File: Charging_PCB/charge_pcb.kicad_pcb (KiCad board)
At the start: 2 copper layers, 96.5 x 50.8 mm, 40 parts, among them J1 PCB_1, J2 Battery, J3 Power Switch, J4 24V Out, J5 Motor_Drive, J6 Motor_Cutter, J7 24V Out, J8 Start, J9 24V out, Q1 BC547C, Q2 IRF9540N, Q3 BC547C, Q4 IRF9540N, U1 INA169

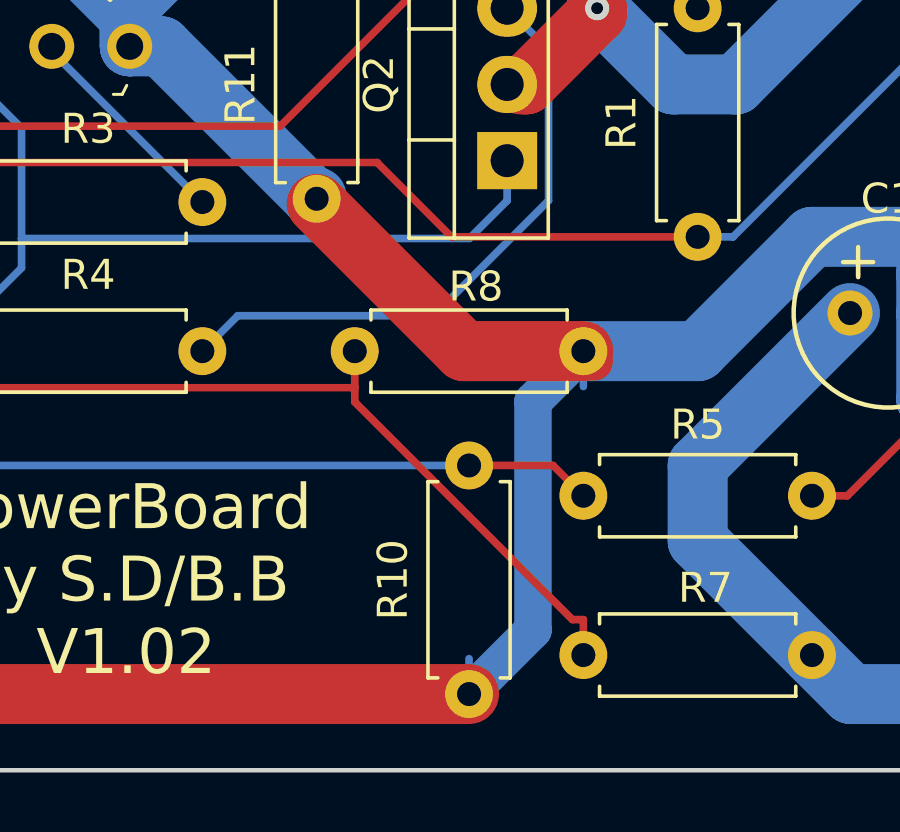
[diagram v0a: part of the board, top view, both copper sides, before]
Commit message: Add Schematic PDF and new Picture
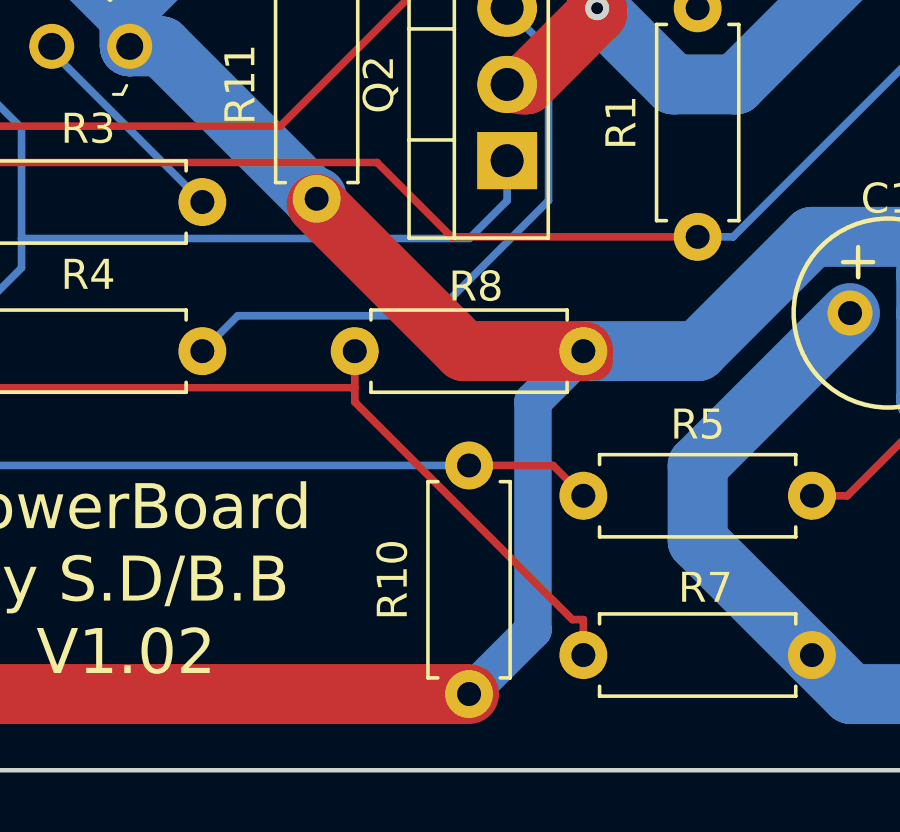
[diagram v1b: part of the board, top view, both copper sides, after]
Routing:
- net GND: track 346.3 -> 333.0 mm
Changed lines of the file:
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@@
   (segment (start 70.360001 114.150001) (end 75.64 119.43) (width 2) (layer "F.Cu") (net 1))
   (segment (start 75.64 119.43) (end 75.64 120.28) (width 2) (layer "F.Cu") (net 1))
-  (segment (start 100.33 140.97) (end 96.52 140.97) (width 1.25) (layer "F.Cu") (net 1))
   (segment (start 145.888671 114.228011) (end 151.25 119.58934) (width 2) (layer "F.Cu") (net 1))
   (segment (start 116.93 124.33) (end 122.0087 129.4087) (width 0.254) (layer "F.Cu") (net 1))
@@
   (segment (start 100.3273 125.2714) (end 101.5487 124.05) (width 0.254) (layer "F.Cu") (net 1))
   (segment (start 130.81 149.86) (end 128.055999 152.614001) (width 2) (layer "F.Cu") (net 1))
-  (segment (start 96.52 140.97) (end 91.44 135.89) (width 1.25) (layer "F.Cu") (net 1))
   (segment (start 75.64 120.28) (end 79.33 123.97) (width 2) (layer "F.Cu") (net 1))
   (segment (start 100.33 140.97) (end 96.34739 140.97) (width 2) (layer "F.Cu") (net 1))
@@
   (segment (start 122.0087 129.4087) (end 122.0087 129.54) (width 0.254) (layer "F.Cu") (net 1))
   (segment (start 157.265999 111.404001) (end 157.265999 120.435999) (width 2) (layer "F.Cu") (net 1))
-  (segment (start 96.52 152.4) (end 96.52 151.2187) (width 0.254) (layer "B.Cu") (net 1))
   (segment (start 98.650999 150.269001) (end 96.52 152.4) (width 1.25) (layer "B.Cu") (net 1))
   (segment (start 85.21 130.81) (end 85.21 129.45) (width 2) (layer "B.Cu") (net 1))
@@
   (segment (start 116.8 147.61) (end 116.8 149.86) (width 2) (layer "B.Cu") (net 1))
   (segment (start 98.650999 142.649001) (end 98.650999 150.269001) (width 1.25) (layer "B.Cu") (net 1))
-  (segment (start 100.33 140.97) (end 100.33 142.1513) (width 0.254) (layer "B.Cu") (net 1))
   (segment (start 104.14 140.97) (end 107.95 137.16) (width 2) (layer "B.Cu") (net 1))
   (segment (start 159.79 149.86) (end 160.75 150.82) (width 2) (layer "B.Cu") (net 1))
